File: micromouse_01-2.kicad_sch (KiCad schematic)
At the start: 50 parts, among them IC3 ADS7066IRTER, IC4 PCA9632TK,118, J2 Fan+, J3 Fan-, J4 Battery, Q1 SiA910, Q2 Q_PMOS_GSD, Q3 Q_PMOS_GSD, Q4 Q_PMOS_GSD, SW1 SSSS810701, U4 SMT-0440-S-R, U5 WS2812-2020, U6 MCP73831-2-OT, U7 LXDC55FAAA-203

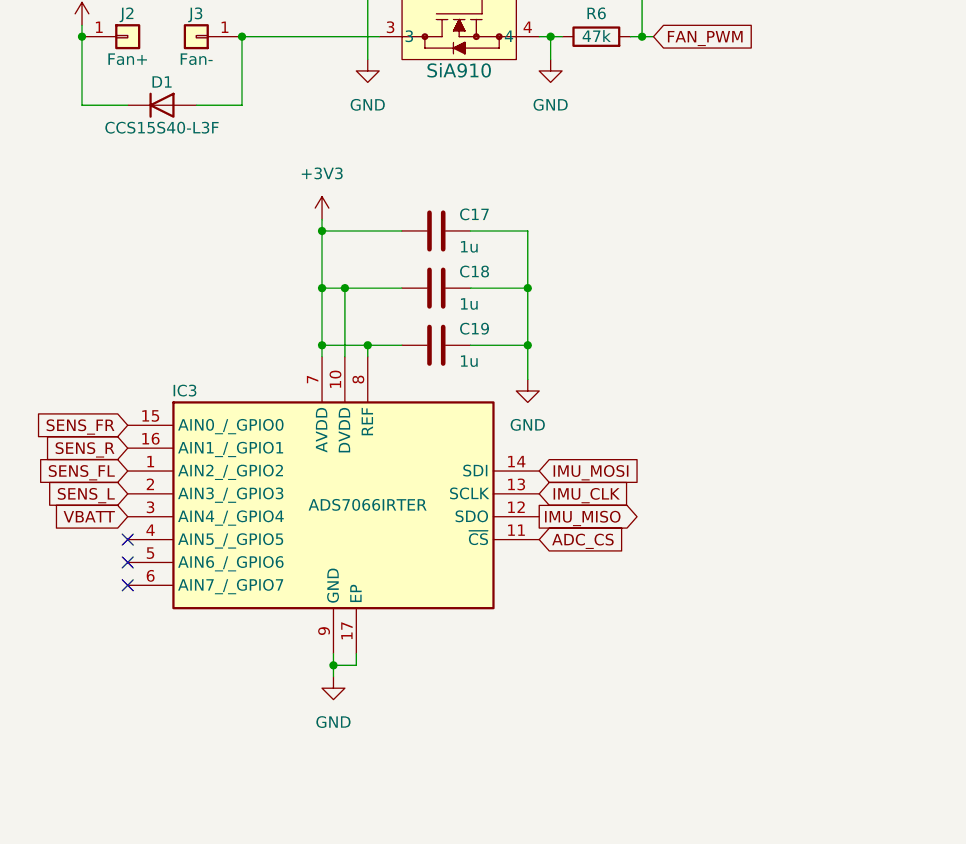
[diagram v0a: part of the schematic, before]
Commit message: 新しい部品乗せた
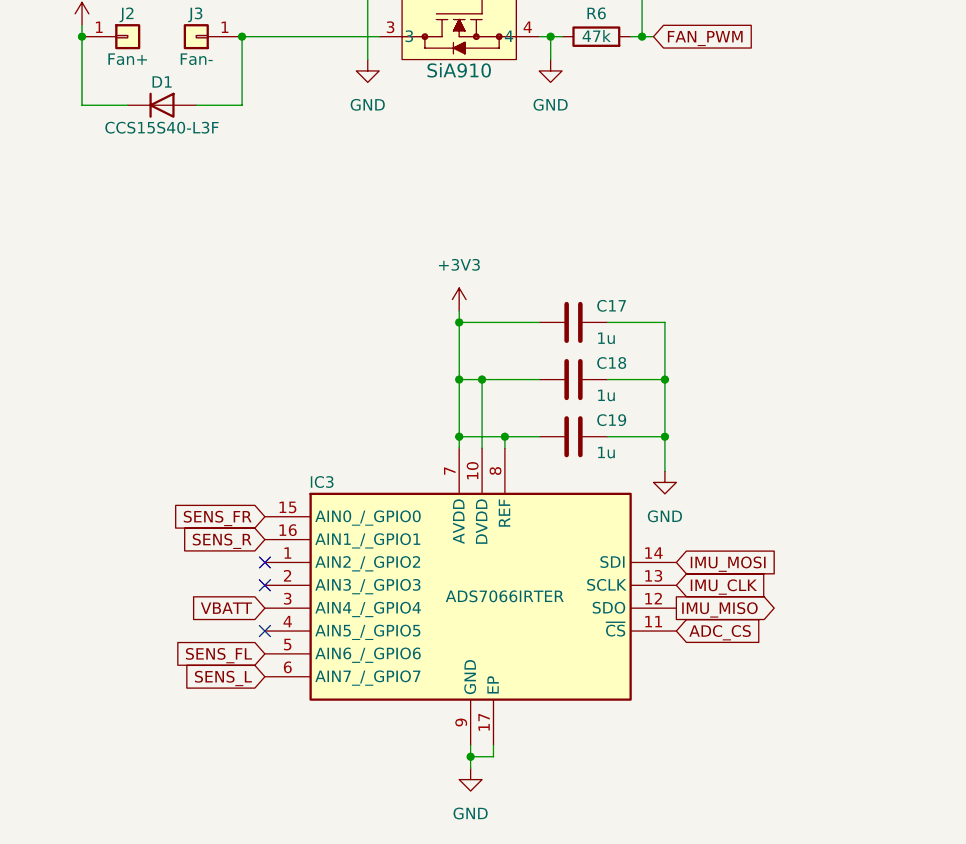
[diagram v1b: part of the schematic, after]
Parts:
- J4: footprint (none) -> footprints:MK06-4.5
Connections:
- net SENS_FL: now also IC3.5 (AIN6_/_GPIO6); no longer IC3.1 (AIN2_/_GPIO2)
- net SENS_L: now also IC3.6 (AIN7_/_GPIO7); no longer IC3.2 (AIN3_/_GPIO3)
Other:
- moved on the sheet: C17, C18, C19, IC3
